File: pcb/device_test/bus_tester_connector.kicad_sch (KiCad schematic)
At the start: 6 parts, among them J301 USB_C_Receptacle_USB2.0_16P, J302 Conn_02x10_Row_Letter_First

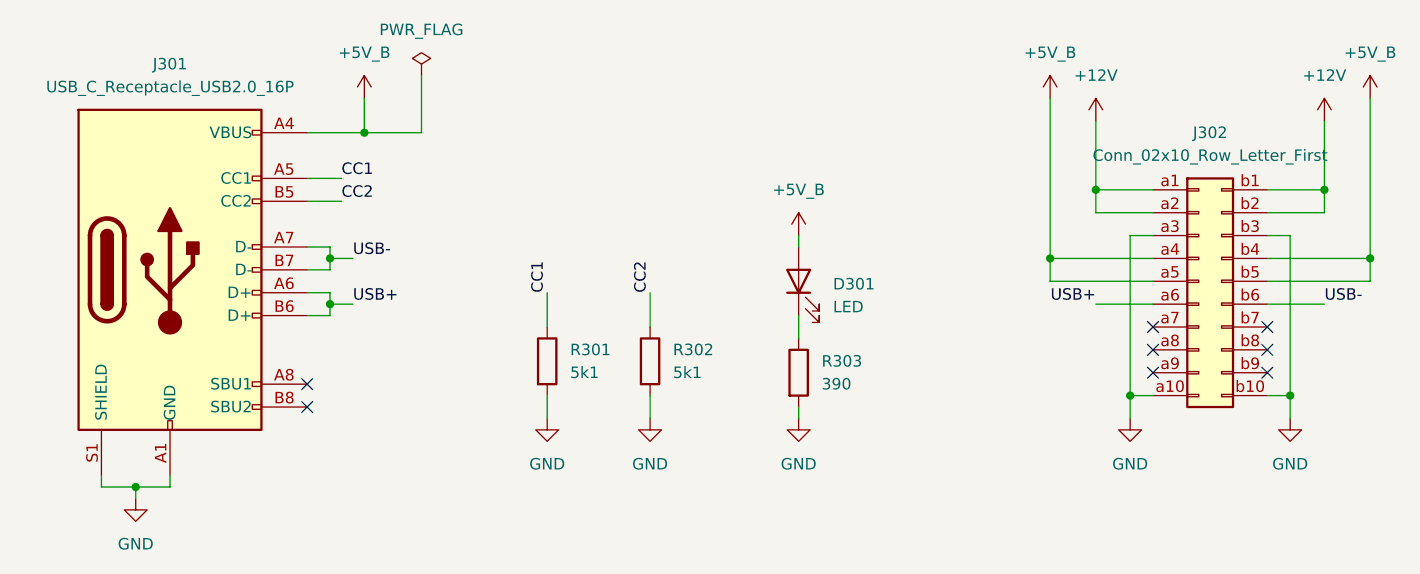
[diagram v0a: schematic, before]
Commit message: update
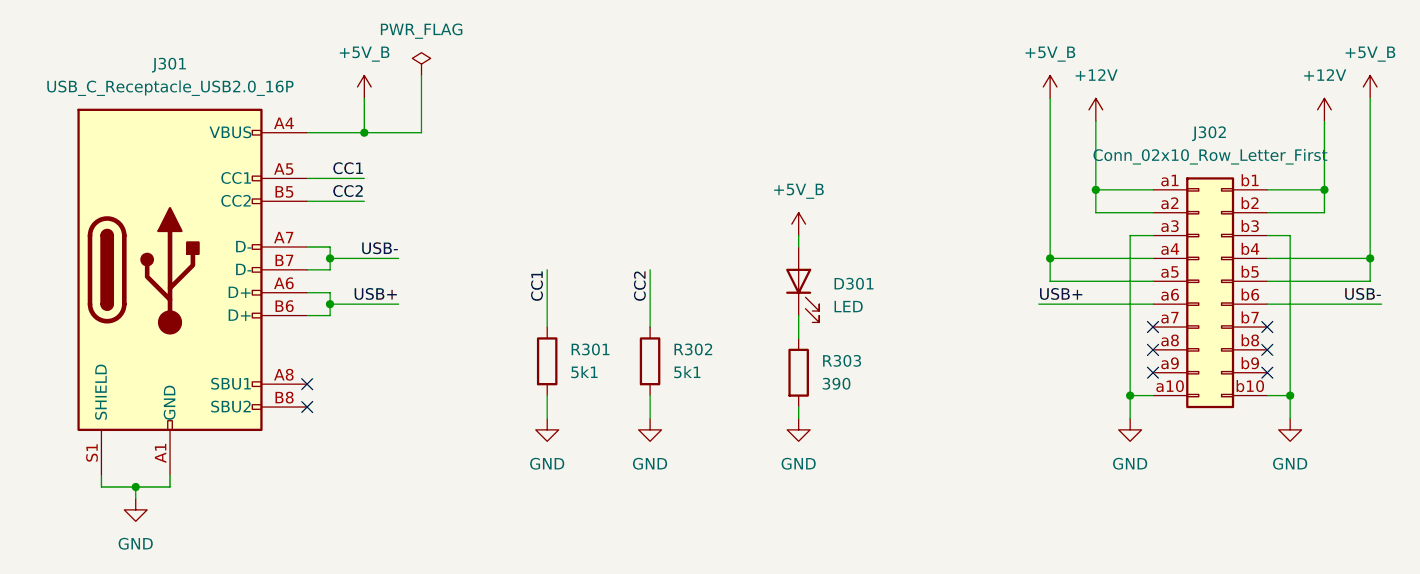
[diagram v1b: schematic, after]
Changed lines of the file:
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@@
 	(wire
 		(pts
-			(xy 195.58 90.17) (xy 201.93 90.17)
+			(xy 195.58 90.17) (xy 208.28 90.17)
 		)
 		(stroke
@@
 	(wire
 		(pts
-			(xy 91.44 90.17) (xy 93.98 90.17)
+			(xy 91.44 90.17) (xy 99.06 90.17)
 		)
 		(stroke
@@
 	(wire
 		(pts
-			(xy 127 88.9) (xy 127 92.71)
+			(xy 127 86.36) (xy 127 92.71)
 		)
 		(stroke
@@
 	(wire
 		(pts
-			(xy 176.53 90.17) (xy 182.88 90.17)
+			(xy 170.18 90.17) (xy 182.88 90.17)
 		)
 		(stroke
@@
 	(wire
 		(pts
-			(xy 91.44 85.09) (xy 93.98 85.09)
+			(xy 91.44 85.09) (xy 99.06 85.09)
 		)
 		(stroke
@@
 	(wire
 		(pts
-			(xy 88.9 78.74) (xy 92.71 78.74)
+			(xy 88.9 78.74) (xy 95.25 78.74)
 		)
 		(stroke
@@
 	(wire
 		(pts
-			(xy 88.9 76.2) (xy 92.71 76.2)
-		)
-		(stroke
-			(width 0)
-			(type default)
-		)
-	)
-	(wire
-		(pts
-			(xy 115.57 88.9) (xy 115.57 92.71)
+			(xy 88.9 76.2) (xy 95.25 76.2)
+		)
+		(stroke
+			(width 0)
+			(type default)
+		)
+	)
+	(wire
+		(pts
+			(xy 115.57 86.36) (xy 115.57 92.71)
 		)
 		(stroke
@@
 	)
 	(label "USB-"
-		(at 201.93 90.17 0)
+		(at 208.28 90.17 180)
+		(effects
+			(font
+				(size 1.27 1.27)
+			)
+			(justify right bottom)
+		)
+	)
+	(label "CC2"
+		(at 127 86.36 270)
+		(effects
+			(font
+				(size 1.27 1.27)
+			)
+			(justify right bottom)
+		)
+	)
+	(label "USB-"
+		(at 99.06 85.09 180)
+		(effects
+			(font
+				(size 1.27 1.27)
+			)
+			(justify right bottom)
+		)
+	)
+	(label "CC1"
+		(at 115.57 86.36 270)
+		(effects
+			(font
+				(size 1.27 1.27)
+			)
+			(justify right bottom)
+		)
+	)
+	(label "CC1"
+		(at 95.25 76.2 180)
+		(effects
+			(font
+				(size 1.27 1.27)
+			)
+			(justify right bottom)
+		)
+	)
+	(label "USB+"
+		(at 170.18 90.17 0)
 		(effects
 			(font
@@
 		)
 	)
+	(label "USB+"
+		(at 99.06 90.17 180)
+		(effects
+			(font
+				(size 1.27 1.27)
+			)
+			(justify right bottom)
+		)
+	)
 	(label "CC2"
-		(at 127 88.9 90)
-		(effects
-			(font
-				(size 1.27 1.27)
-			)
-			(justify left bottom)
-		)
-	)
-	(label "USB-"
-		(at 93.98 85.09 0)
-		(effects
-			(font
-				(size 1.27 1.27)
-			)
-			(justify left bottom)
-		)
-	)
-	(label "CC1"
-		(at 115.57 88.9 90)
-		(effects
-			(font
-				(size 1.27 1.27)
-			)
-			(justify left bottom)
-		)
-	)
-	(label "CC1"
-		(at 92.71 76.2 0)
-		(effects
-			(font
-				(size 1.27 1.27)
-			)
-			(justify left bottom)
-		)
-	)
-	(label "USB+"
-		(at 176.53 90.17 180)
-		(effects
-			(font
-				(size 1.27 1.27)
-			)
-			(justify right bottom)
-		)
-	)
-	(label "USB+"
-		(at 93.98 90.17 0)
-		(effects
-			(font
-				(size 1.27 1.27)
-			)
-			(justify left bottom)
-		)
-	)
-	(label "CC2"
-		(at 92.71 78.74 0)
-		(effects
-			(font
-				(size 1.27 1.27)
-			)
-			(justify left bottom)
-		)
-	)
+		(at 95.25 78.74 180)
+		(effects
+			(font
+				(size 1.27 1.27)
+			)
+			(justify right bottom)
+		)
+	)
